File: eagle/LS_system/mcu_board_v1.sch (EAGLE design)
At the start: 24 parts, among them IC2 LT1763CS8-3.3, IC3 STM32F4XX_64, Q2 PFET, X1 USBSMD, X2 MURDOCK_STACK

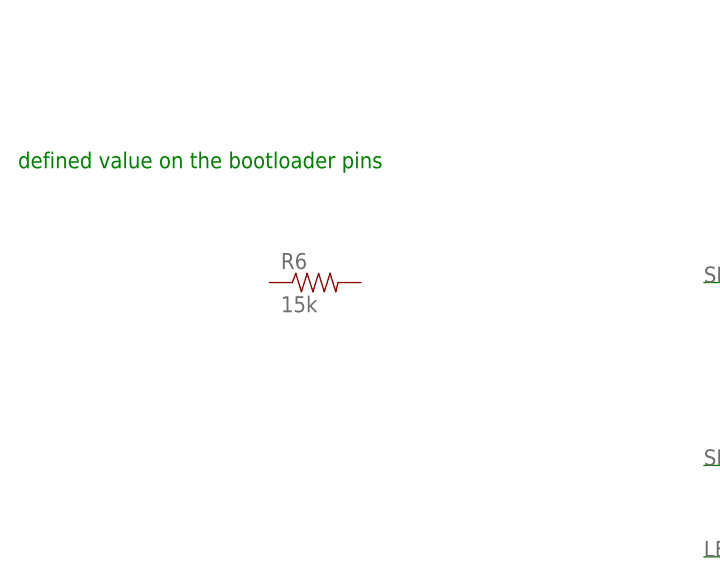
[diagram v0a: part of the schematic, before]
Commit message: typo
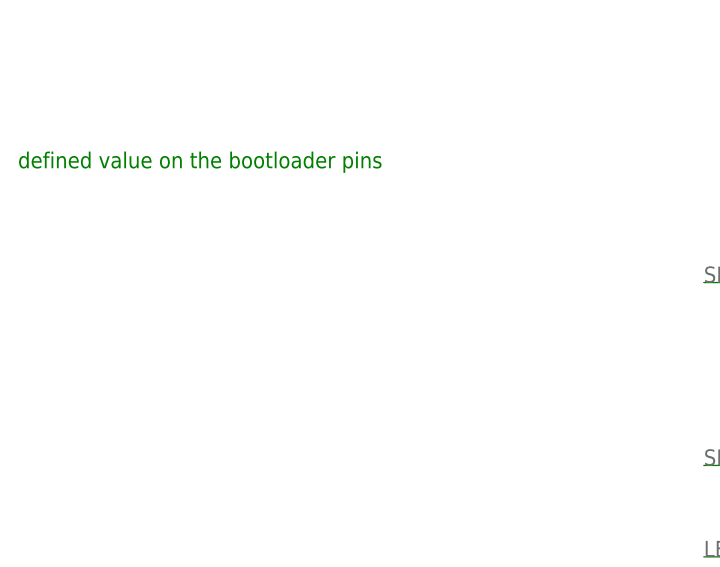
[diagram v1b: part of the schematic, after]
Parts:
- removed R6: 15k, SparkFun-Resistors:RESISTOR0402-RES
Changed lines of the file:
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@@
 <part name="R5" library="SparkFun-Resistors" deviceset="RESISTOR" device="0402-RES" value="15k"/>
 <part name="GND3" library="SparkFun-Aesthetics" deviceset="GND" device=""/>
-<part name="R6" library="SparkFun-Resistors" deviceset="RESISTOR" device="0402-RES" value="15k"/>
 </parts>
 <sheets>
@@
 <instance part="R5" gate="G$1" x="-86.36" y="111.76" rot="R90"/>
 <instance part="GND3" gate="1" x="-86.36" y="104.14" smashed="yes"/>
-<instance part="R6" gate="G$1" x="-60.96" y="48.26"/>
 </instances>
 <busses>
